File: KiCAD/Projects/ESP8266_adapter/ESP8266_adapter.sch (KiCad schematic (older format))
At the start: 14 parts, among them P1 PWR, P2 CONN_LEFT, P3 CONN_RIGHT, P4 UART_PROG, P5 PWR, P6 PWR, SW1 RST_SWITCH, U1 NCP1117DT33G_MountingTab, U2 ESP-12E

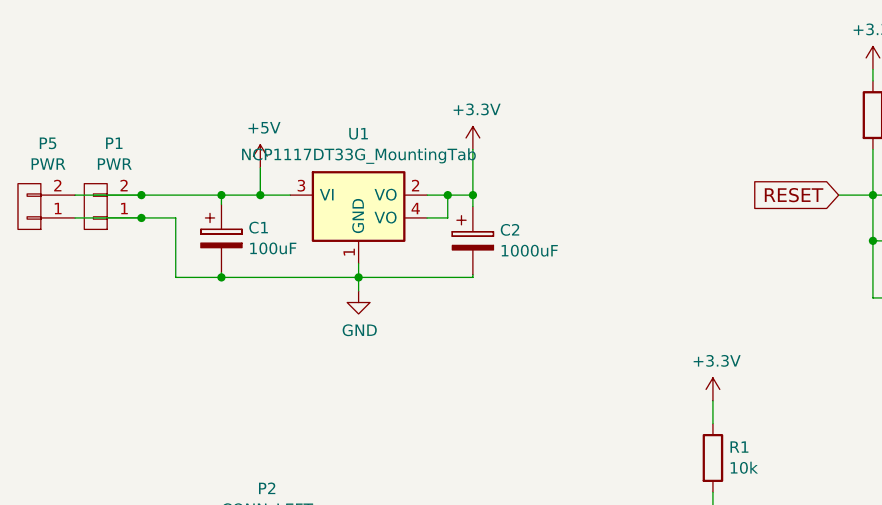
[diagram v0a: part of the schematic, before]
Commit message: Update with minor modifications
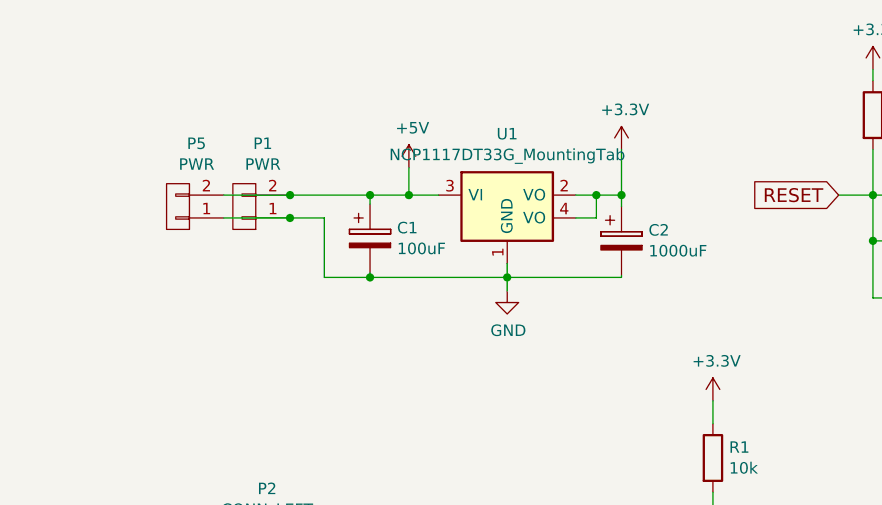
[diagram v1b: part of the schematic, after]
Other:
- moved on the sheet: C1, C2, P1, P5, U1
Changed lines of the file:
@@
 LIBS:zetex
 LIBS:Zilog
-LIBS:ESP8266
-LIBS:mq_snsr
-LIBS:tgs2602
 LIBS:ESP8266_adapter-cache
 EELAYER 26 0
@@
 L CONN_01X02 P1
 U 1 1 58A34B8F
-P 1750 2250
-F 0 "P1" H 1669 1975 50  0000 C CNN
-F 1 "PWR" H 1669 2066 50  0000 C CNN
-F 2 "Connectors_Phoenix:PhoenixContact_MCV-G_02x5.08mm_Vertical" H 1750 2250 50  0001 C CNN
-F 3 "" H 1750 2250 50  0000 C CNN
-	1    1750 2250
+P 2400 2250
+F 0 "P1" H 2319 1975 50  0000 C CNN
+F 1 "PWR" H 2319 2066 50  0000 C CNN
+F 2 "Connectors_Phoenix:PhoenixContact_MCV-G_02x5.08mm_Vertical" H 2400 2250 50  0001 C CNN
+F 3 "" H 2400 2250 50  0000 C CNN
+	1    2400 2250
 	-1   0    0    1
 $EndComp
@@
 L CP C2
 U 1 1 58A35C0B
-P 3400 2400
-F 0 "C2" H 3518 2446 50  0000 L CNN
-F 1 "1000uF" H 3518 2355 50  0000 L CNN
-F 2 "Capacitors_THT:CP_Radial_D5.0mm_P2.50mm" H 3438 2250 50  0001 C CNN
-F 3 "" H 3400 2400 50  0000 C CNN
-	1    3400 2400
+P 4050 2400
+F 0 "C2" H 4168 2446 50  0000 L CNN
+F 1 "1000uF" H 4168 2355 50  0000 L CNN
+F 2 "Capacitors_THT:CP_Radial_D5.0mm_P2.50mm" H 4088 2250 50  0001 C CNN
+F 3 "" H 4050 2400 50  0000 C CNN
+	1    4050 2400
 	1    0    0    -1
 $EndComp
@@
 L +3.3V #PWR01
 U 1 1 58A3656F
-P 3400 2000
-F 0 "#PWR01" H 3400 1850 50  0001 C CNN
-F 1 "+3.3V" H 3415 2173 50  0000 C CNN
-F 2 "" H 3400 2000 50  0000 C CNN
-F 3 "" H 3400 2000 50  0000 C CNN
-	1    3400 2000
+P 4050 2000
+F 0 "#PWR01" H 4050 1850 50  0001 C CNN
+F 1 "+3.3V" H 4065 2173 50  0000 C CNN
+F 2 "" H 4050 2000 50  0000 C CNN
+F 3 "" H 4050 2000 50  0000 C CNN
+	1    4050 2000
 	1    0    0    -1
 $EndComp
@@
 L CONN_01X02 P5
 U 1 1 58A41395
-P 1460 2250
-F 0 "P5" H 1379 1975 50  0000 C CNN
-F 1 "PWR" H 1379 2066 50  0000 C CNN
-F 2 "Pin_Headers:Pin_Header_Straight_1x02_Pitch2.54mm" H 1460 2250 50  0001 C CNN
-F 3 "" H 1460 2250 50  0000 C CNN
-	1    1460 2250
+P 2110 2250
+F 0 "P5" H 2029 1975 50  0000 C CNN
+F 1 "PWR" H 2029 2066 50  0000 C CNN
+F 2 "Pin_Headers:Pin_Header_Straight_1x02_Pitch2.54mm" H 2110 2250 50  0001 C CNN
+F 3 "" H 2110 2250 50  0000 C CNN
+	1    2110 2250
 	-1   0    0    1
 $EndComp
@@
 L CP C1
 U 1 1 58A35C63
-P 2300 2390
-F 0 "C1" H 2418 2436 50  0000 L CNN
-F 1 "100uF" H 2418 2345 50  0000 L CNN
-F 2 "Capacitors_THT:CP_Radial_D5.0mm_P2.50mm" H 2338 2240 50  0001 C CNN
-F 3 "" H 2300 2390 50  0000 C CNN
-	1    2300 2390
+P 2950 2390
+F 0 "C1" H 3068 2436 50  0000 L CNN
+F 1 "100uF" H 3068 2345 50  0000 L CNN
+F 2 "Capacitors_THT:CP_Radial_D5.0mm_P2.50mm" H 2988 2240 50  0001 C CNN
+F 3 "" H 2950 2390 50  0000 C CNN
+	1    2950 2390
 	1    0    0    -1
 $EndComp
@@
 L +5V #PWR010
 U 1 1 58A5288A
-P 2470 2080
-F 0 "#PWR010" H 70  -170 50  0001 C CNN
-F 1 "+5V" H 2485 2253 50  0000 C CNN
-F 2 "" H 70  -20 50  0001 C CNN
-F 3 "" H 70  -20 50  0001 C CNN
-	1    2470 2080
+P 3120 2080
+F 0 "#PWR010" H 720 -170 50  0001 C CNN
+F 1 "+5V" H 3135 2253 50  0000 C CNN
+F 2 "" H 720 -20 50  0001 C CNN
+F 3 "" H 720 -20 50  0001 C CNN
+	1    3120 2080
 	1    0    0    -1
 $EndComp
@@
 Connection ~ 5150 2200
 Wire Wire Line
-	3200 2200 3400 2200
-Wire Wire Line
-	3400 2000 3400 2250
-Connection ~ 3400 2200
+	3850 2200 4050 2200
+Wire Wire Line
+	4050 2000 4050 2250
+Connection ~ 4050 2200
 Wire Wire Line
 	6450 2950 6450 2800
@@
 Connection ~ 7700 4550
 Wire Wire Line
-	1660 2200 2600 2200
-Wire Wire Line
-	1660 2300 2100 2300
-Wire Wire Line
-	2100 2300 2100 2560
-Wire Wire Line
-	2100 2560 3400 2560
-Connection ~ 1950 2300
+	2310 2200 3250 2200
+Wire Wire Line
+	2310 2300 2750 2300
+Wire Wire Line
+	2750 2300 2750 2560
+Wire Wire Line
+	2750 2560 4050 2560
+Connection ~ 2600 2300
 Wire Wire Line
 	6600 2500 6850 2500
 Wire Wire Line
-	2300 2240 2300 2200
-Connection ~ 2300 2200
-Connection ~ 1950 2200
-Wire Wire Line
-	2470 2080 2470 2200
-Connection ~ 2470 2200
-Wire Wire Line
-	3400 2560 3400 2550
-Wire Wire Line
-	2900 2500 2900 2620
-Connection ~ 2900 2560
+	2950 2240 2950 2200
+Connection ~ 2950 2200
+Connection ~ 2600 2200
+Wire Wire Line
+	3120 2080 3120 2200
+Connection ~ 3120 2200
+Wire Wire Line
+	4050 2560 4050 2550
+Wire Wire Line
+	3550 2500 3550 2620
+Connection ~ 3550 2560
 $Comp
 L GND #PWR011
 U 1 1 58A537AF
-P 2900 2620
-F 0 "#PWR011" H 2900 2370 50  0001 C CNN
-F 1 "GND" H 2905 2447 50  0000 C CNN
-F 2 "" H 2900 2620 50  0000 C CNN
-F 3 "" H 2900 2620 50  0000 C CNN
-	1    2900 2620
-	1    0    0    -1
-$EndComp
-Wire Wire Line
-	2300 2540 2300 2560
-Connection ~ 2300 2560
+P 3550 2620
+F 0 "#PWR011" H 3550 2370 50  0001 C CNN
+F 1 "GND" H 3555 2447 50  0000 C CNN
+F 2 "" H 3550 2620 50  0000 C CNN
+F 3 "" H 3550 2620 50  0000 C CNN
+	1    3550 2620
+	1    0    0    -1
+$EndComp
+Wire Wire Line
+	2950 2540 2950 2560
+Connection ~ 2950 2560
 $Comp
 L NCP1117DT33G_MountingTab U1
 U 1 1 58A544EF
-P 2900 2200
-F 0 "U1" H 2900 2467 50  0000 C CNN
-F 1 "NCP1117DT33G_MountingTab" H 2900 2376 50  0000 C CNN
-F 2 "TO_SOT_Packages_SMD:SOT-223" H 210 380 50  0001 L CNN
-F 3 "" H 160 630 50  0001 C CNN
-	1    2900 2200
-	1    0    0    -1
-$EndComp
-Wire Wire Line
-	3200 2300 3290 2300
-Wire Wire Line
-	3290 2300 3290 2200
-Connection ~ 3290 2200
+P 3550 2200
+F 0 "U1" H 3550 2467 50  0000 C CNN
+F 1 "NCP1117DT33G_MountingTab" H 3550 2376 50  0000 C CNN
+F 2 "TO_SOT_Packages_SMD:SOT-223" H 860 380 50  0001 L CNN
+F 3 "" H 810 630 50  0001 C CNN
+	1    3550 2200
+	1    0    0    -1
+$EndComp
+Wire Wire Line
+	3850 2300 3940 2300
+Wire Wire Line
+	3940 2300 3940 2200
+Connection ~ 3940 2200
 $EndSCHEMATC
